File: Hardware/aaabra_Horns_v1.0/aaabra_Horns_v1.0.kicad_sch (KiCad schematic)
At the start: 17 parts, among them J1 Conn_01x03, J2 Conn_01x02, J3 Conn_01x02, J4 Conn_01x02, Q1 IRFR010PBF

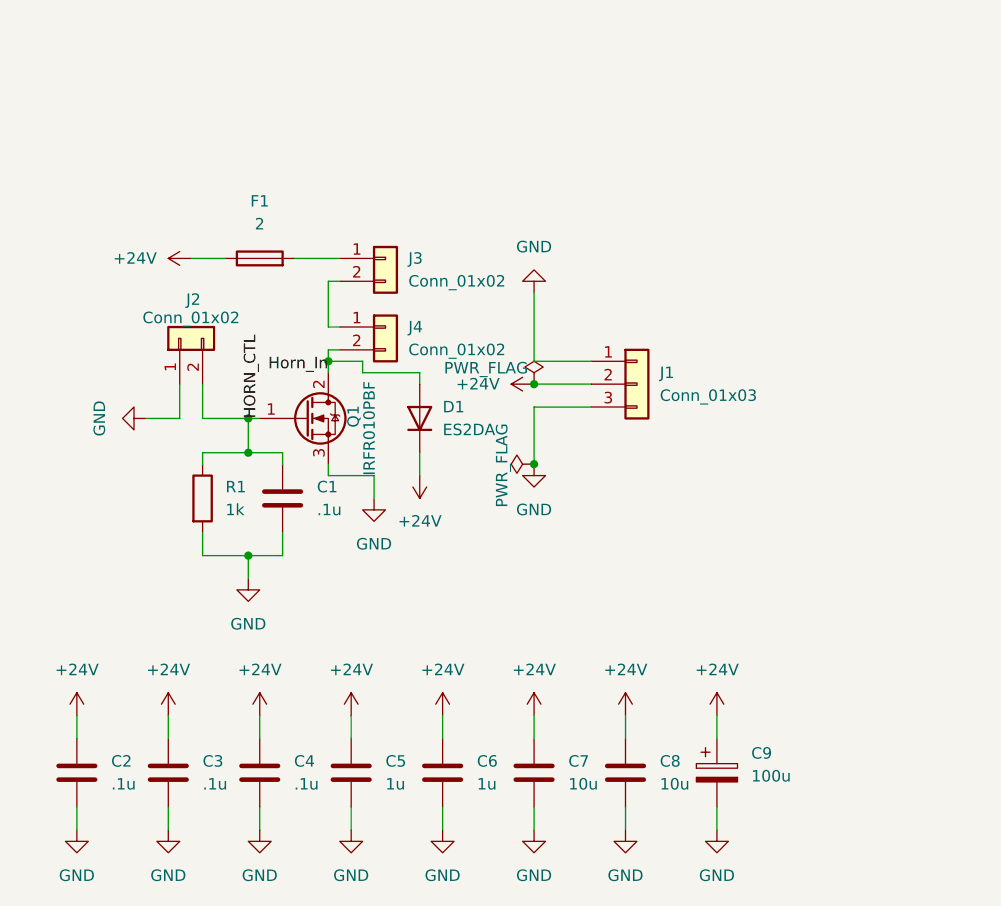
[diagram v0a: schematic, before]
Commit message: onboarding
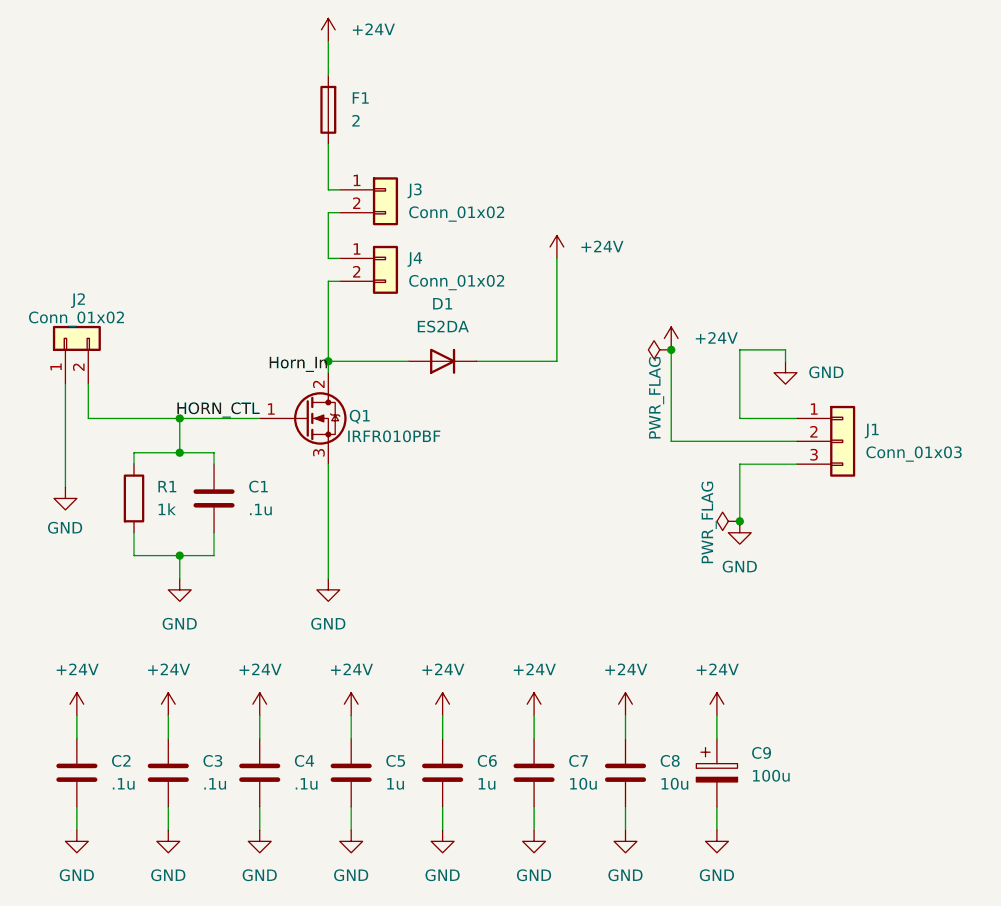
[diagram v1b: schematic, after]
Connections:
- net +24V: now also F1.2; no longer F1.1
- net at J3.1 (Pin_1): now also F1.1; no longer F1.2
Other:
- moved on the sheet: C1, D1, F1, J1, J2, J3, J4, R1
